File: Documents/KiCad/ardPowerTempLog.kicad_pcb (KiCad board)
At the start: 2 copper layers, 36 parts, among them J1 R1, J10 5-pin_3-pole_3,5mm_audio_head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, J11 4-pin_3LED_header, J12 Conn_01x02_Male, J13 Conn_01x02_Male, J2 S2, J3 T3, J4 OneWire bus, J5 LED sensor, J6 5-pin_3-pole_3,5mm_audio_head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, J7 5-pin_3-pole_3,5mm_audio_head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, J8 5-pin_3-pole_3,5mm_audio_head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, J9 5-pin_3-pole_3,5mm_audio_head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, Q1 Q_Photo_NPN_CBE, U1 DS18B20

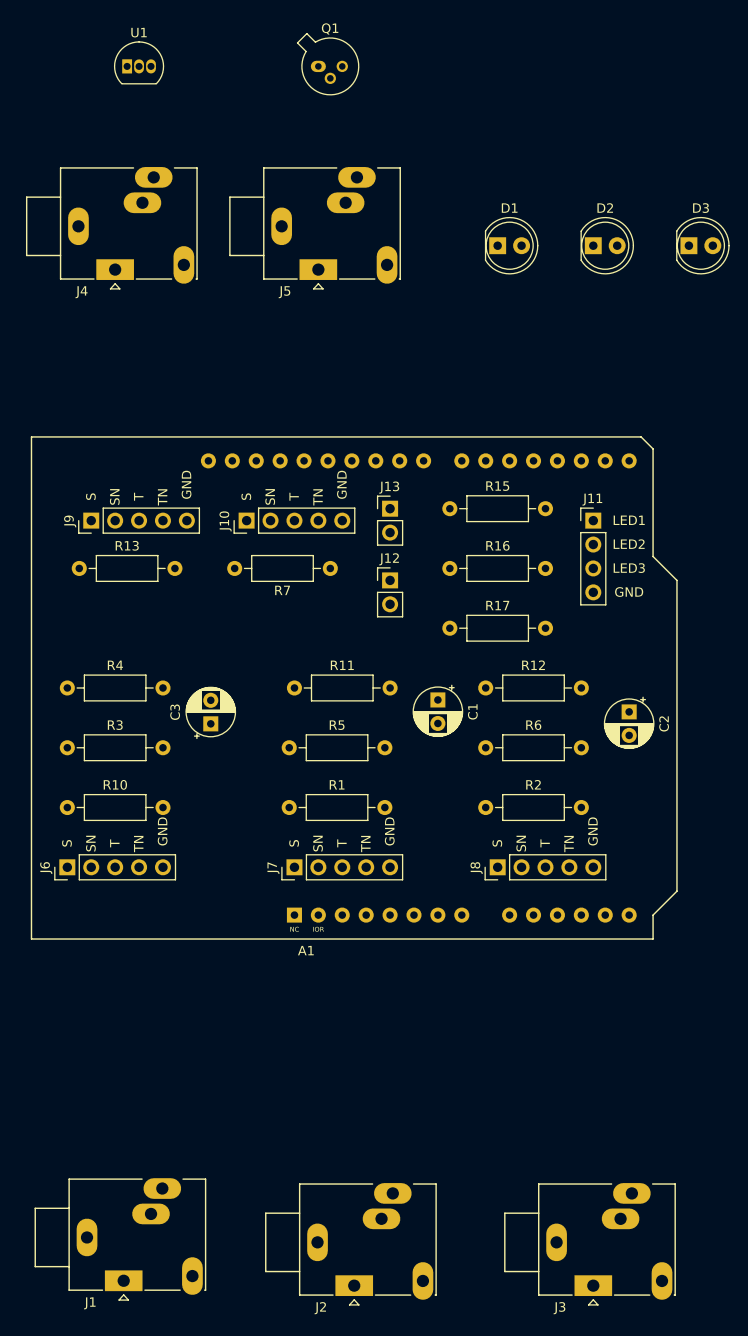
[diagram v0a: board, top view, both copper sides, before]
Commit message: schematics
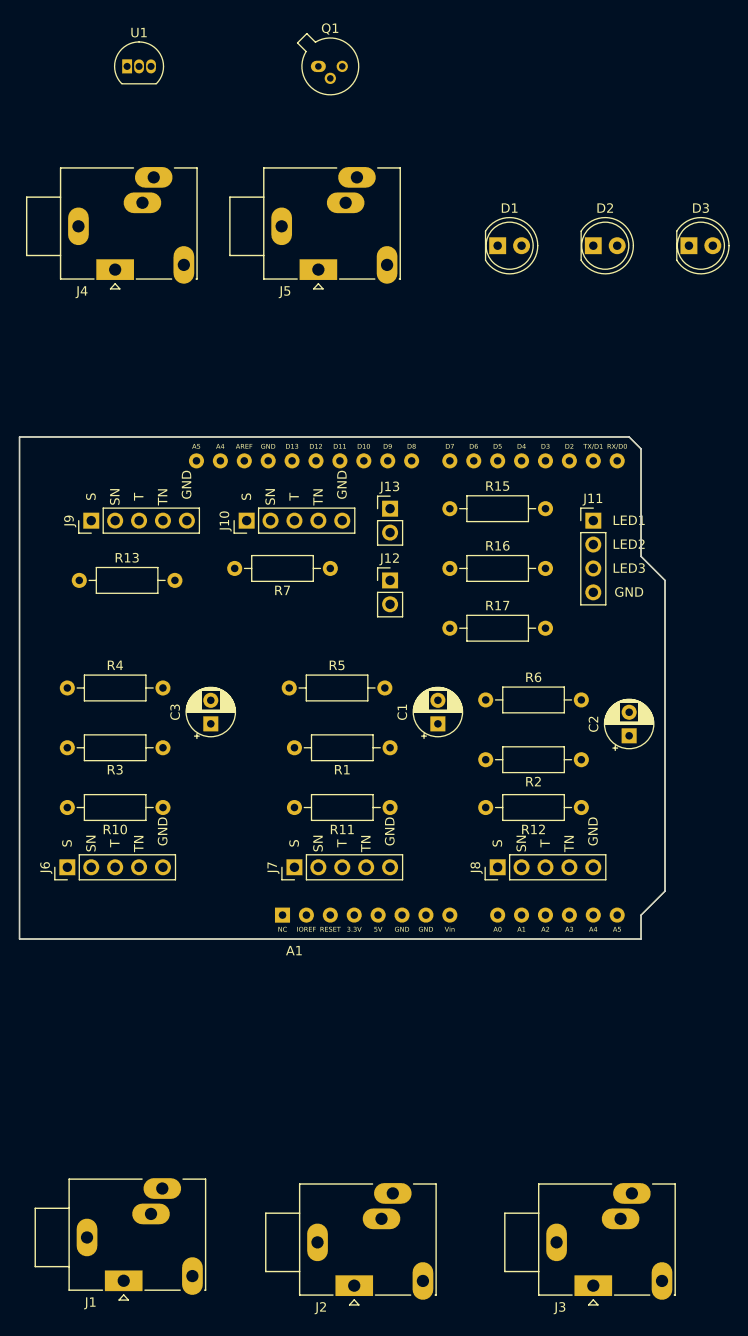
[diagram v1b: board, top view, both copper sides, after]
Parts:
- R6: value 100k -> 10k
- moved R11 16.3 mm to (144.8, 97.8), turned to 180 degrees
- moved R12 16.3 mm to (165.1, 97.8), turned to 180 degrees
- moved R1 12.5 mm to (144.8, 91.4), turned to 180 degrees
- moved R2 11.4 mm to (165.1, 92.7), turned to 180 degrees
- moved R10 10.2 mm to (120.7, 97.8), turned to 180 degrees
- moved R3 10.2 mm to (120.7, 91.4), turned to 180 degrees
- moved R5 6.35 mm to (134.1, 85.1)
- moved R6 5.08 mm to (154.9, 86.4)
- moved C1 2.54 mm to (149.9, 88.9), turned to 90 degrees
- moved C2 2.54 mm to (170.2, 90.2), turned to 90 degrees
- moved A1 1.27 mm to (133.3, 109.2)
- moved R13 1.27 mm to (111.8, 73.7)
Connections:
- J1 pad T: Net-(A1-Pad11) -> Net-(A1-Pad10)
- J12 pad 2: Net-(A1-Pad10) -> Net-(A1-Pad32)
- J2 pad T: Net-(A1-Pad12) -> Net-(A1-Pad11)
- J3 pad T: Net-(A1-Pad13) -> Net-(A1-Pad12)
- J6 pad 3: Net-(A1-Pad11) -> Net-(A1-Pad10)
- J7 pad 3: Net-(A1-Pad12) -> Net-(A1-Pad11)
- J8 pad 3: Net-(A1-Pad13) -> Net-(A1-Pad12)
- R10 pad 1: Net-(A1-Pad11) -> Net-(A1-Pad10)
- R11 pad 1: Net-(A1-Pad12) -> Net-(A1-Pad11)
- R12 pad 1: Net-(A1-Pad13) -> Net-(A1-Pad12)
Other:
- board outline added: 68.6 x 53.3 mm
